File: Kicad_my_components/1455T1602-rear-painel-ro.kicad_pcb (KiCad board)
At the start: 2 copper layers, 165 x 51.5 mm, 1 part

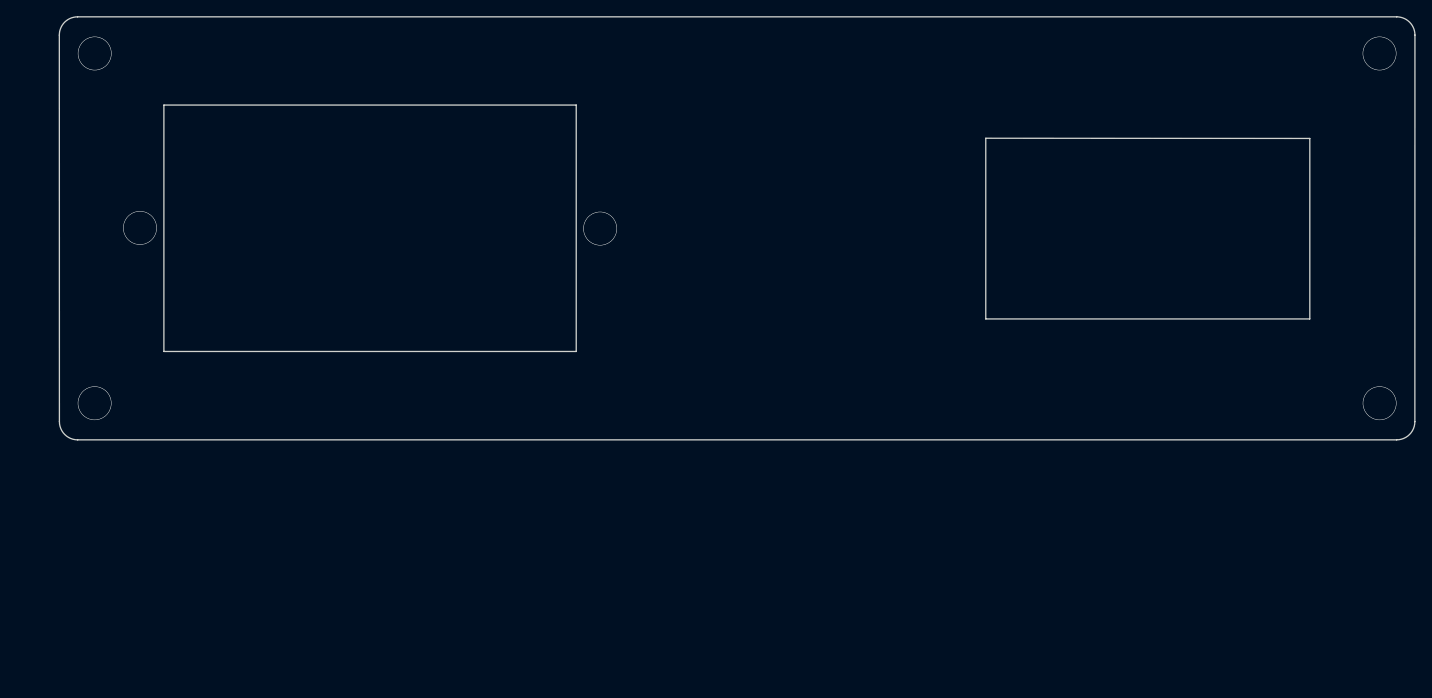
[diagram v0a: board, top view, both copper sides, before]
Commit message: Fixed all
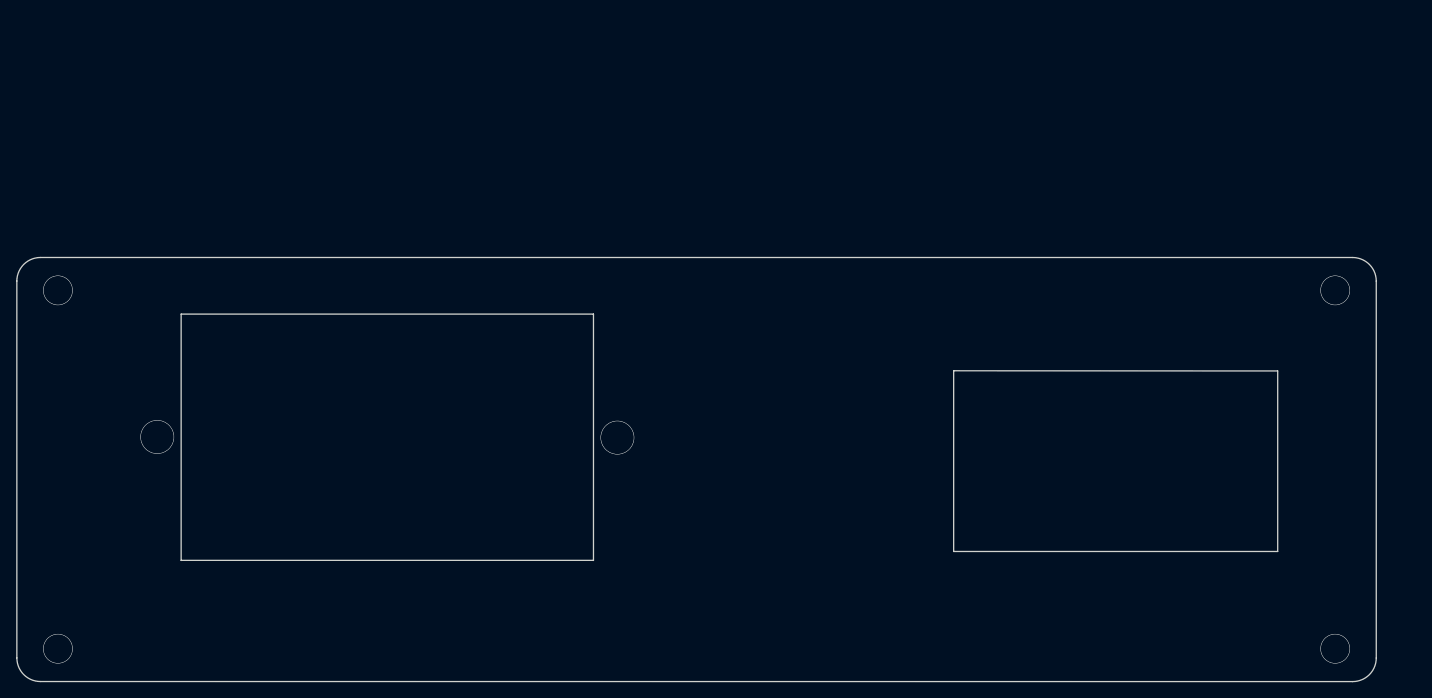
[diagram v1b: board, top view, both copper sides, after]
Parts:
- moved ? 28.6 mm to (215.1, 113.6)
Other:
- board size 165 x 51.5 mm -> 165.5 x 51.6 mm
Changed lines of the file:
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@@
   (net 0 "")
   (footprint "clipboard:39385a36-6dcb-40a6-94e9-d8d4c5d5e346" (layer "F.Cu")
-    (at 218.98 85.3)
+    (at 215.07 113.61)
     (fp_text reference "" (at 0 0) (layer "F.SilkS")
       (effects (font (size 1.27 1.27) (thickness 0.15)))
@@
     (fp_line (start 0 0) (end 0 -21.975) (layer "Edge.Cuts") (width 0.12))
   )
-  (gr_line (start 129.67 59.26) (end 129.67 89.26) (layer "Edge.Cuts") (width 0.1))
-  (gr_line (start 68.97009 100.02) (end 229.54991 100.02) (layer "Edge.Cuts") (width 0.1))
-  (gr_arc (start 231.76991 97.8) (mid 231.119687 99.369777) (end 229.54991 100.02) (layer "Edge.Cuts") (width 0.1))
-  (gr_line (start 79.47 89.26) (end 79.47 59.26) (layer "Edge.Cuts") (width 0.1))
-  (gr_arc (start 229.55991 48.52) (mid 231.129751 49.170249) (end 231.78 50.74009) (layer "Edge.Cuts") (width 0.1))
-  (gr_arc (start 68.97009 100.02) (mid 67.400313 99.369777) (end 66.75009 97.8) (layer "Edge.Cuts") (width 0.1))
-  (gr_line (start 68.96009 48.52) (end 229.55991 48.52) (layer "Edge.Cuts") (width 0.1))
-  (gr_line (start 79.47 59.26) (end 129.67 59.26) (layer "Edge.Cuts") (width 0.1))
-  (gr_line (start 231.77991 50.74) (end 231.76991 97.8) (layer "Edge.Cuts") (width 0.1))
-  (gr_arc (start 66.74 50.74009) (mid 67.390249 49.170249) (end 68.96009 48.52) (layer "Edge.Cuts") (width 0.1))
-  (gr_line (start 66.75009 97.8) (end 66.74009 50.74) (layer "Edge.Cuts") (width 0.1))
-  (gr_line (start 129.67 89.26) (end 79.47 89.26) (layer "Edge.Cuts") (width 0.1))
-  (segment (start 227.47 95.55009) (end 227.48 95.56009) (width 0.25) (layer "F.Cu") (net 0))
-  (via (at 71.04 95.56009) (size 4.1) (drill 4) (layers "F.Cu" "B.Cu") (free) (net 0))
-  (via (at 132.58 74.3) (size 4.1) (drill 4) (layers "F.Cu" "B.Cu") (free) (net 0))
-  (via (at 227.48 95.56009) (size 4.1) (drill 4) (layers "F.Cu" "B.Cu") (free) (net 0))
-  (via (at 227.47 52.98) (size 4.1) (drill 4) (layers "F.Cu" "B.Cu") (free) (net 0))
-  (via (at 76.56 74.22) (size 4.1) (drill 4) (layers "F.Cu" "B.Cu") (free) (net 0))
-  (via (at 71.05 52.98) (size 4.1) (drill 4) (layers "F.Cu" "B.Cu") (free) (net 0))
-  (segment (start 71.05 95.55009) (end 71.04 95.56009) (width 0.25) (layer "B.Cu") (net 0))
+  (gr_line (start 131.77 84.71) (end 131.77 114.71) (layer "Edge.Cuts") (width 0.1))
+  (gr_line (start 224.197058 129.45) (end 64.442942 129.442942) (layer "Edge.Cuts") (width 0.1))
+  (gr_line (start 227.07 80.692942) (end 227.07 126.577058) (layer "Edge.Cuts") (width 0.1))
+  (gr_arc (start 227.07 126.577058) (mid 226.228535 128.608535) (end 224.197058 129.45) (layer "Edge.Cuts") (width 0.1))
+  (gr_arc (start 64.442942 129.442942) (mid 62.411465 128.601477) (end 61.57 126.57) (layer "Edge.Cuts") (width 0.1))
+  (gr_line (start 81.57 114.71) (end 81.57 84.71) (layer "Edge.Cuts") (width 0.1))
+  (gr_arc (start 224.197058 77.82) (mid 226.228535 78.661465) (end 227.07 80.692942) (layer "Edge.Cuts") (width 0.1))
+  (gr_line (start 81.57 84.71) (end 131.77 84.71) (layer "Edge.Cuts") (width 0.1))
+  (gr_line (start 64.44 77.817058) (end 224.197058 77.82) (layer "Edge.Cuts") (width 0.1))
+  (gr_line (start 131.77 114.69) (end 81.57 114.69) (layer "Edge.Cuts") (width 0.1))
+  (gr_arc (start 61.567058 80.69) (mid 62.408523 78.658523) (end 64.44 77.817058) (layer "Edge.Cuts") (width 0.1))
+  (gr_line (start 61.57 126.57) (end 61.567058 80.69) (layer "Edge.Cuts") (width 0.1))
+  (via (at 134.68 99.75) (size 4.1) (drill 4) (layers "F.Cu" "B.Cu") (free) (net 0))
+  (via (at 222.07 125.45) (size 3.6) (drill 3.5) (layers "F.Cu" "B.Cu") (free) (net 0))
+  (via (at 78.66 99.67) (size 4.1) (drill 4) (layers "F.Cu" "B.Cu") (free) (net 0))
+  (via (at 222.07 81.82) (size 3.6) (drill 3.5) (layers "F.Cu" "B.Cu") (free) (net 0))
+  (via (at 66.57 81.82) (size 3.6) (drill 3.5) (layers "F.Cu" "B.Cu") (free) (net 0))
+  (via (at 66.57 125.45) (size 3.6) (drill 3.5) (layers "F.Cu" "B.Cu") (free) (net 0))
 )
